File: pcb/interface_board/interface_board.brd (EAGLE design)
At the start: 72 x 56 mm, 55 parts, among them IC1 V7805-1000, K1 61400416021, U1 SFW15R-1STE1LF, U2 SFW15R-1STE1LF, U3 DMG1012T, U4 TENDA_P200, U5 PAM2306AYPKE

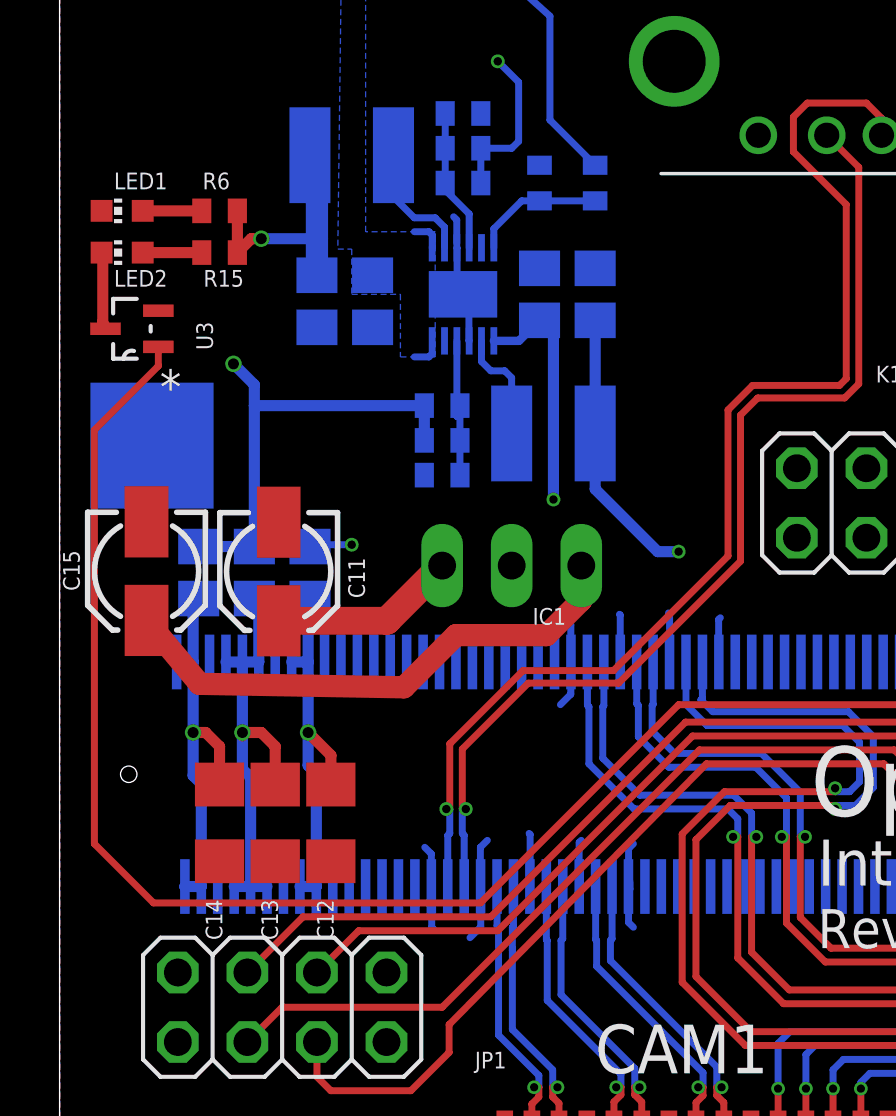
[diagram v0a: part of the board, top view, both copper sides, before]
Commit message: tune
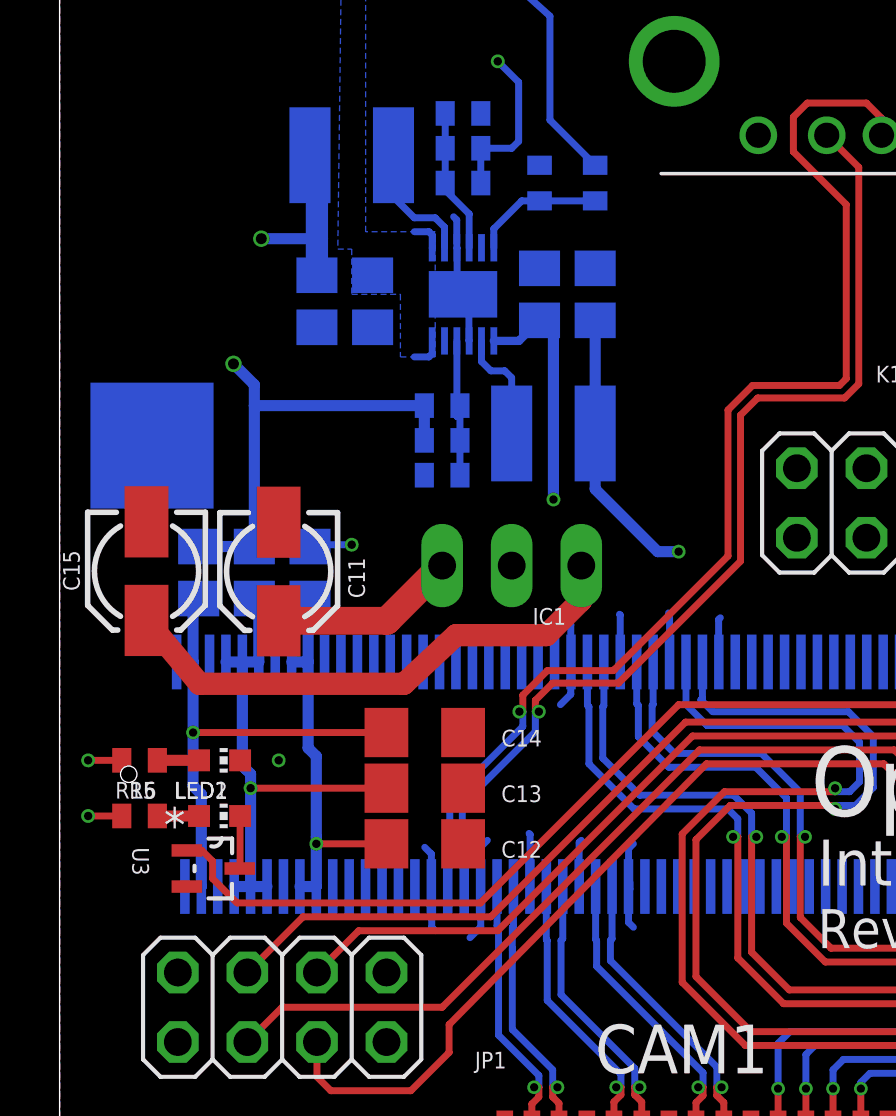
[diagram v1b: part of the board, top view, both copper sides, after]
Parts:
- moved LED2 20.9 mm to (5.84, 18.0), turned to 270 degrees
- moved R15 20.8 mm to (2.92, 18.0), turned to 0 degrees
- moved LED1 20.4 mm to (5.84, 20.1), turned to 270 degrees
- moved R6 20.3 mm to (2.92, 20.1), turned to 0 degrees
- moved U3 19.9 mm to (5.61, 16.1), turned to 0 degrees
- moved C14 8.19 mm to (13.3, 21.1), turned to 0 degrees
- moved C13 5.61 mm to (13.3, 19.1), turned to 0 degrees
- moved C12 3.51 mm to (13.3, 17.0), turned to 0 degrees
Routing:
- net GPIO47_1V8: track 61.4 -> 39.2 mm
- net CM_VBAT: track 14.5 -> 19.0 mm
- net CM_3V3: track 16.0 -> 18.1 mm
- net N$33: track 2.80 -> 1.92 mm
- net N$9: track 2.16 -> 1.52 mm
- net N$32: track 2.16 -> 1.52 mm
- net USB_D_N: track 43.3 -> 42.7 mm
- net USB_D_P: track 38.0 -> 37.5 mm
- net +3V3: track 189.9 -> 189.8 mm, vias 4 -> 6
- net GND: track 40.2 -> 40.3 mm, vias 0 -> 1
